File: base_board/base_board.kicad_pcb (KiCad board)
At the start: 6 copper layers, 50 x 50 mm, 56 parts, among them J1 Conn_ARM_JTAG_SWD_20, SW1 SW_Push, U1 STM32F446ZEJx, U2 IS42S16400J-xT, U3 BMI270, U4 USB_C_Receptacle_USB2.0, U5 10p, U6 10p, U7 LD3985M33R_SOT23, Y1 Crystal_GND24

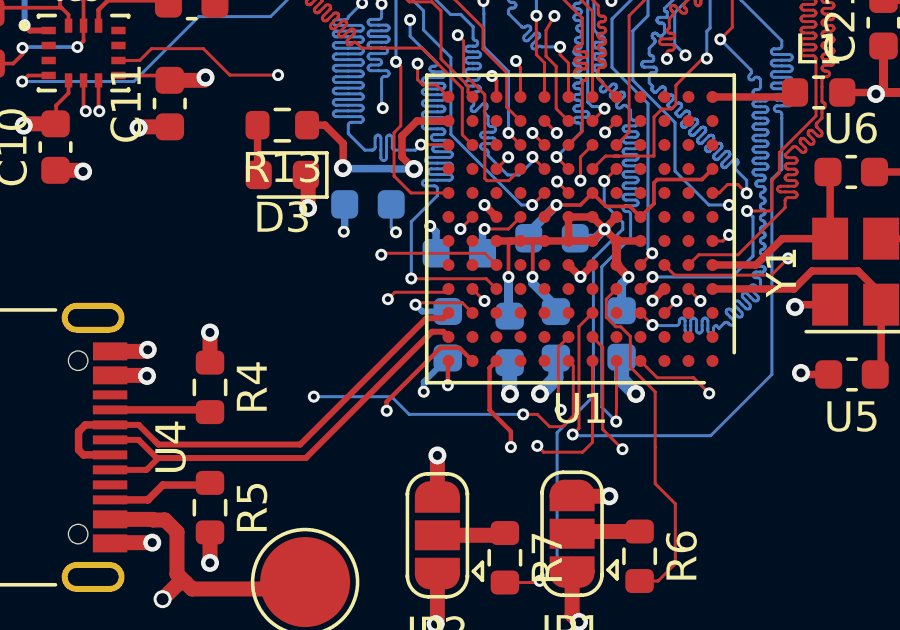
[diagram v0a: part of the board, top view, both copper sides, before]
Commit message: [pcb] added review corrections
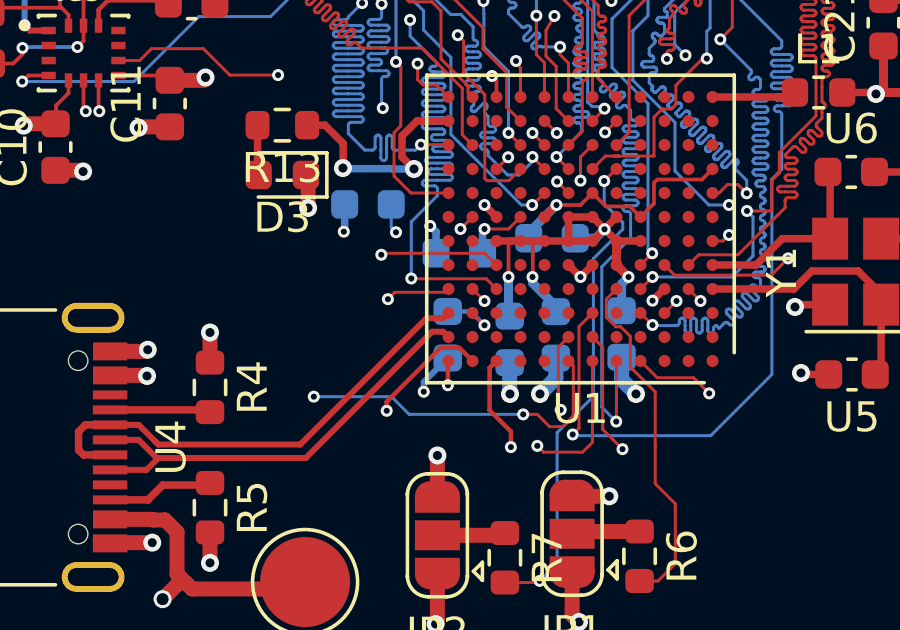
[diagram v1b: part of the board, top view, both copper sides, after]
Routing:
- net /FMC_A0: track 32.3 -> 21.5 mm
- net /SWO: track 70.9 -> 66.5 mm
- net +3V3: track 78.0 -> 76.8 mm
- net /FMC_A6: track 36.2 -> 35.7 mm
